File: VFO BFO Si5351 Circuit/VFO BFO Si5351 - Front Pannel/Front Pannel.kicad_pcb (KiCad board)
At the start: 2 copper layers, 149.4 x 69.2 mm, 23 parts, among them J1 LED, J2 Optical Rotary Encoder, J3 Mecc_rotary encoder, J4 VFO_Front_Pannel, SW1 RotaryEncoder_Clarifier, SW2 SW_Band, SW3 SW_Mode, SW4 SW_AGC, SW5 SW_ATT, SW6 SW_Scan, SW7 SW_Step, SW8 SW_RTTY_CW, U1 Ili9341_Module_TFT_320x240_To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

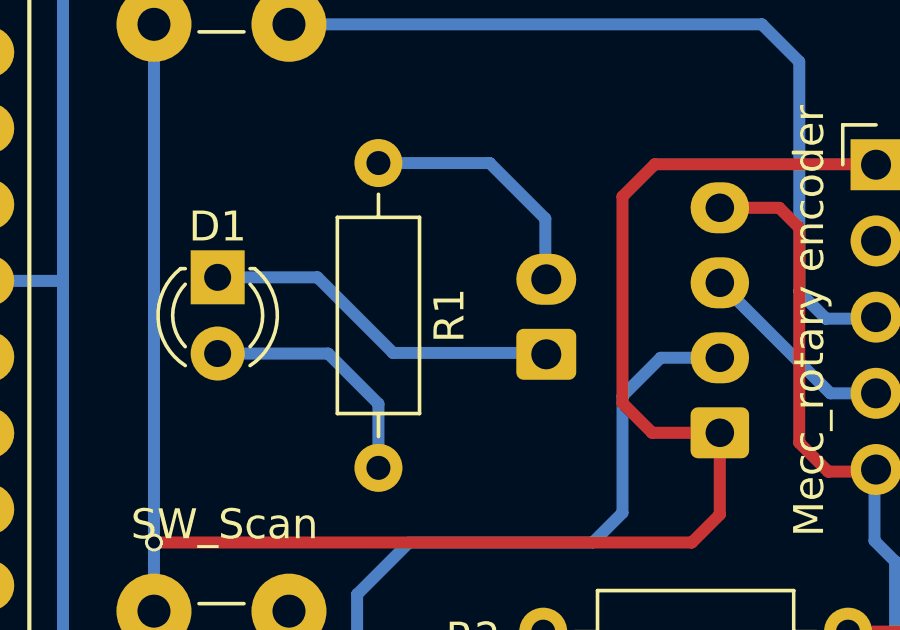
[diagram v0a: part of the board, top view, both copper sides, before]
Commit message: ultimato PCB
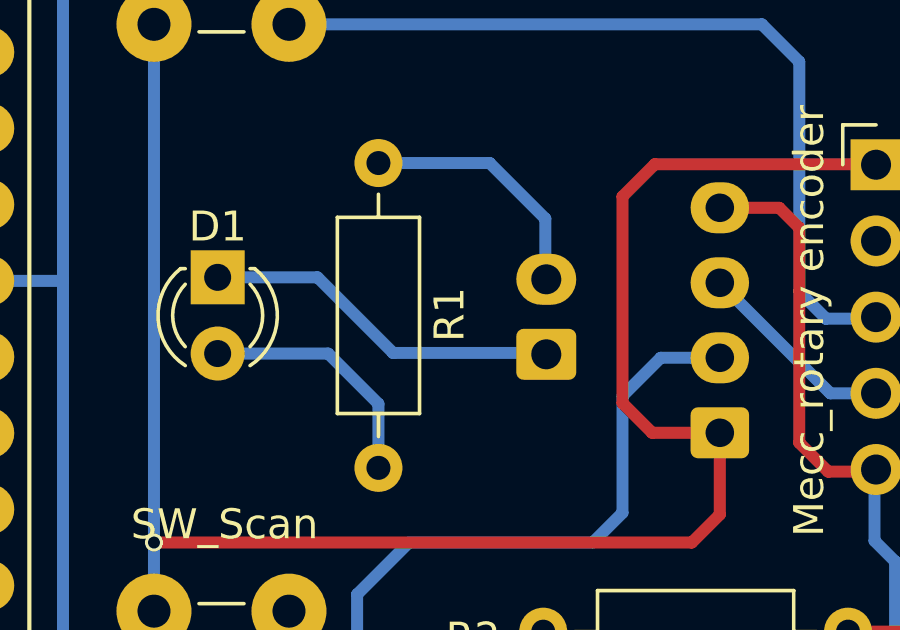
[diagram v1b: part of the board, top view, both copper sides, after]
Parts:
- R2, R3: value 10K -> 4.7K
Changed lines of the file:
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@@
 			)
 		)
-		(property "Value" "10K"
-			(at 5.08 2.37 0)
+		(property "Value" "4.7K"
+			(at 14.956 -0.3708 0)
 			(layer "F.Fab")
 			(effects
@@
 			)
 		)
-		(property "Value" "10K"
-			(at 5.08 2.37 0)
+		(property "Value" "4.7K"
+			(at 14.956 -0.0708 0)
 			(layer "F.Fab")
 			(effects
@@
 		(tags "Resistor Axial_DIN0207 series Axial Horizontal pin pitch 10.16mm 0.25W = 1/4W length 6.3mm diameter 2.5mm")
 		(property "Reference" "R1"
-			(at 5.08 -2.37 90)
+			(at 5.0502 -2.37 90)
 			(layer "F.SilkS")
 			(effects
@@
 		)
 		(property "Value" "R=Vled-2/20mA"
-			(at 5.08 2.37 90)
+			(at 4.8006 2.1274 90)
 			(layer "F.Fab")
 			(effects
 				(font
-					(size 1 1)
+					(size 0.6 0.8)
 					(thickness 0.15)
 				)
@@
 		(tags "tact sw push 6mm")
 		(property "Reference" "SW8"
-			(at 3.22 7.502 180)
+			(at 3.22 6.9252 180)
 			(layer "F.Fab")
 			(effects
